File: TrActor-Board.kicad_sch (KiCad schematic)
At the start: 24 parts, among them J3 GCT4720, J4 Batt, J5 NTC, SW1 Power, SW2 Reset, U3 ICM-40609, U6 USBLC6-2P6

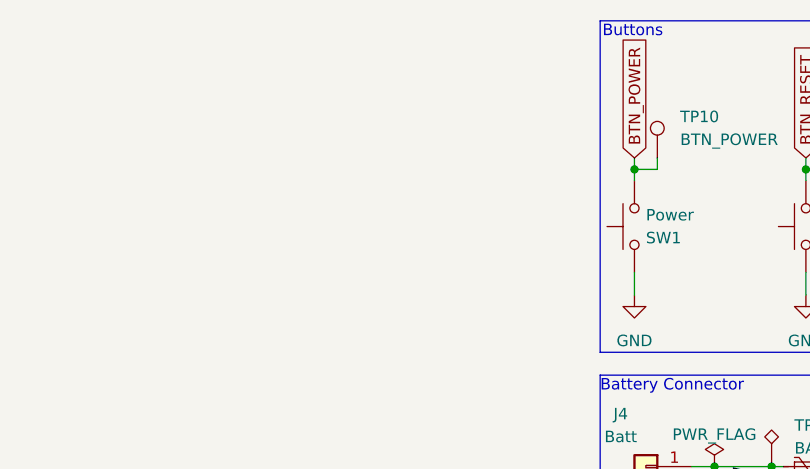
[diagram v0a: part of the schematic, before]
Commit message: mag added. ready for order?
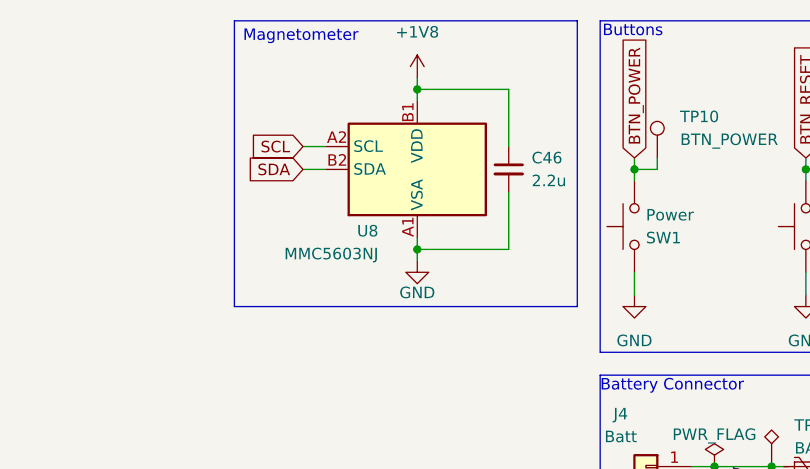
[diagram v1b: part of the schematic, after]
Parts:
- added C46: 2.2u, Capacitor_SMD:C_0603_1608Metric, symbol Device:C_Small
- added U8: MMC5603NJ, Package_BGA:WLP-4_0.86x0.86mm_P0.4mm, symbol Sensor_Magnetic:MMC5633NJL
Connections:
- net +1V8: now also C46.1, U8.B1 (VDD)
- net GND: now also C46.2, U8.A1 (VSA)
- new net SCL: U8.A2 (SCL)
- new net SDA: U8.B2 (SDA)
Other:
- note added: "Magnetometer"

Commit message: ordering commit fr
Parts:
- TP10, TP11, TP12, TP22, TP23, TP5, TP9: now left out of the parts list
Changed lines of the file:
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@@
 		(body_style 1)
 		(exclude_from_sim no)
-		(in_bom yes)
+		(in_bom no)
 		(on_board yes)
 		(in_pos_files yes)
@@
 		(body_style 1)
 		(exclude_from_sim no)
-		(in_bom yes)
+		(in_bom no)
 		(on_board yes)
 		(in_pos_files yes)
@@
 		(body_style 1)
 		(exclude_from_sim no)
-		(in_bom yes)
+		(in_bom no)
 		(on_board yes)
 		(in_pos_files yes)
@@
 		(body_style 1)
 		(exclude_from_sim no)
-		(in_bom yes)
+		(in_bom no)
 		(on_board yes)
 		(in_pos_files yes)
@@
 		(body_style 1)
 		(exclude_from_sim no)
-		(in_bom yes)
+		(in_bom no)
 		(on_board yes)
 		(in_pos_files yes)
@@
 		(body_style 1)
 		(exclude_from_sim no)
-		(in_bom yes)
+		(in_bom no)
 		(on_board yes)
 		(in_pos_files yes)
@@
 		(body_style 1)
 		(exclude_from_sim no)
-		(in_bom yes)
+		(in_bom no)
 		(on_board yes)
 		(in_pos_files yes)
